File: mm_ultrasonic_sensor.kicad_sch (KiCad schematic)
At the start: 3 parts, among them U4 HC-SR04

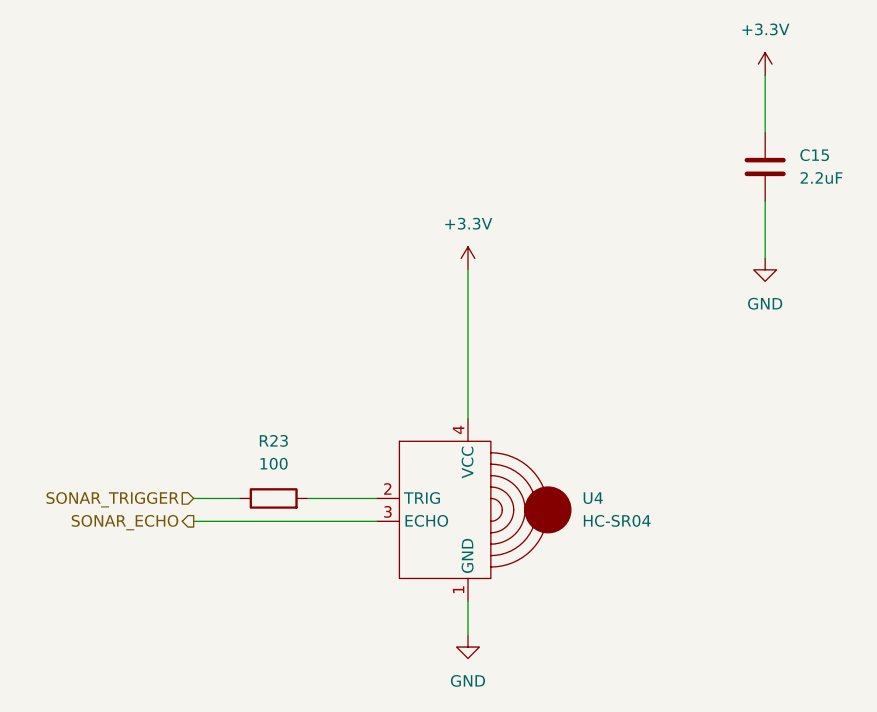
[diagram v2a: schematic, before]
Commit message: dernier tp
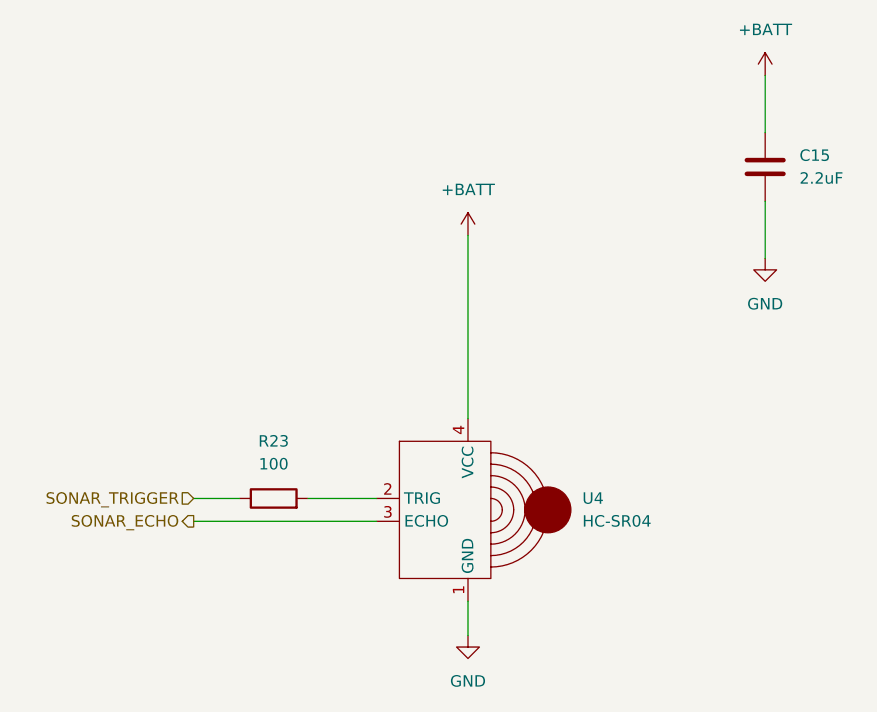
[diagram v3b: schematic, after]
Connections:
- net +3.3V renamed +BATT
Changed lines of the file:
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@@
     (stroke (width 0) (type default))
   )
-  (wire (pts (xy 139.7 63.5) (xy 139.7 80.01))
+  (wire (pts (xy 139.7 59.69) (xy 139.7 80.01))
     (stroke (width 0) (type default))
   )
@@
   (hierarchical_label "SONAR_ECHO" (shape output) (at 109.22 91.44 180) (fields_autoplaced)
     (effects (font (size 1.27 1.27)) (justify right))
+  )
+  (symbol (lib_id "power:+BATT") (at 172.72 41.91 0) (unit 1)
+    (in_bom yes) (on_board yes) (dnp no) (fields_autoplaced)
+    (property "Reference" "#PWR033" (at 172.72 45.72 0)
+      (effects (font (size 1.27 1.27)) hide)
+    )
+    (property "Value" "+BATT" (at 172.72 36.83 0)
+      (effects (font (size 1.27 1.27)))
+    )
+    (property "Footprint" "" (at 172.72 41.91 0)
+      (effects (font (size 1.27 1.27)) hide)
+    )
+    (property "Datasheet" "" (at 172.72 41.91 0)
+      (effects (font (size 1.27 1.27)) hide)
+    )
+    (pin "1")
+    (instances
+      (project "minimouse"
+        (path "/d8fa4cba-2469-4231-847f-065b6b829f44/224298a9-7d6e-4a70-a0a5-f2614895ec28"
+          (reference "#PWR033") (unit 1)
+        )
+      )
+    )
   )
   (symbol (lib_id "power:GND") (at 172.72 62.23 0) (unit 1)
@@
         (path "/d8fa4cba-2469-4231-847f-065b6b829f44/224298a9-7d6e-4a70-a0a5-f2614895ec28"
           (reference "U4") (unit 1)
+        )
+      )
+    )
+  )
+  (symbol (lib_id "power:+BATT") (at 139.7 59.69 0) (unit 1)
+    (in_bom yes) (on_board yes) (dnp no) (fields_autoplaced)
+    (property "Reference" "#PWR040" (at 139.7 63.5 0)
+      (effects (font (size 1.27 1.27)) hide)
+    )
+    (property "Value" "+BATT" (at 139.7 54.61 0)
+      (effects (font (size 1.27 1.27)))
+    )
+    (property "Footprint" "" (at 139.7 59.69 0)
+      (effects (font (size 1.27 1.27)) hide)
+    )
+    (property "Datasheet" "" (at 139.7 59.69 0)
+      (effects (font (size 1.27 1.27)) hide)
+    )
+    (pin "1")
+    (instances
+      (project "minimouse"
+        (path "/d8fa4cba-2469-4231-847f-065b6b829f44/224298a9-7d6e-4a70-a0a5-f2614895ec28"
+          (reference "#PWR040") (unit 1)
         )
       )
@@
         )
       )
-    )
-  )
-  (symbol (lib_id "power:+3.3V") (at 139.7 63.5 0) (unit 1)
-    (in_bom yes) (on_board yes) (dnp no) (fields_autoplaced)
-    (property "Reference" "#PWR033" (at 139.7 67.31 0)
-      (effects (font (size 1.27 1.27)) hide)
-    )
-    (property "Value" "+3.3V" (at 139.7 58.42 0)
-      (effects (font (size 1.27 1.27)))
-    )
-    (property "Footprint" "" (at 139.7 63.5 0)
-      (effects (font (size 1.27 1.27)) hide)
-    )
-    (property "Datasheet" "" (at 139.7 63.5 0)
-      (effects (font (size 1.27 1.27)) hide)
-    )
-    (pin "1")
-    (instances
-      (project "minimouse"
-        (path "/d8fa4cba-2469-4231-847f-065b6b829f44/224298a9-7d6e-4a70-a0a5-f2614895ec28"
-          (reference "#PWR033") (unit 1)
-        )
-      )
-    )
-  )
-  (symbol (lib_id "power:+3.3V") (at 172.72 41.91 0) (unit 1)
-    (in_bom yes) (on_board yes) (dnp no) (fields_autoplaced)
-    (property "Reference" "#PWR035" (at 172.72 45.72 0)
-      (effects (font (size 1.27 1.27)) hide)
-    )
-    (property "Value" "+3.3V" (at 172.72 36.83 0)
-      (effects (font (size 1.27 1.27)))
-    )
-    (property "Footprint" "" (at 172.72 41.91 0)
-      (effects (font (size 1.27 1.27)) hide)
-    )
-    (property "Datasheet" "" (at 172.72 41.91 0)
-      (effects (font (size 1.27 1.27)) hide)
-    )
-    (pin "1")
-    (instances
-      (project "minimouse"
-        (path "/d8fa4cba-2469-4231-847f-065b6b829f44/224298a9-7d6e-4a70-a0a5-f2614895ec28"
-          (reference "#PWR035") (unit 1)
-        )
-      )
